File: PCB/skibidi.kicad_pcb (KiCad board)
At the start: 2 copper layers, 99.5 x 79.5 mm, 18 parts, among them J1 Conn_01x05_Pin, SW1 SW_SPDT, SW2 SW_Push, SW3 SW_Push, SW4 SW_Push, SW5 SW_Push, SW6 SW_Push, U1 XIAO-RP2040-DIP

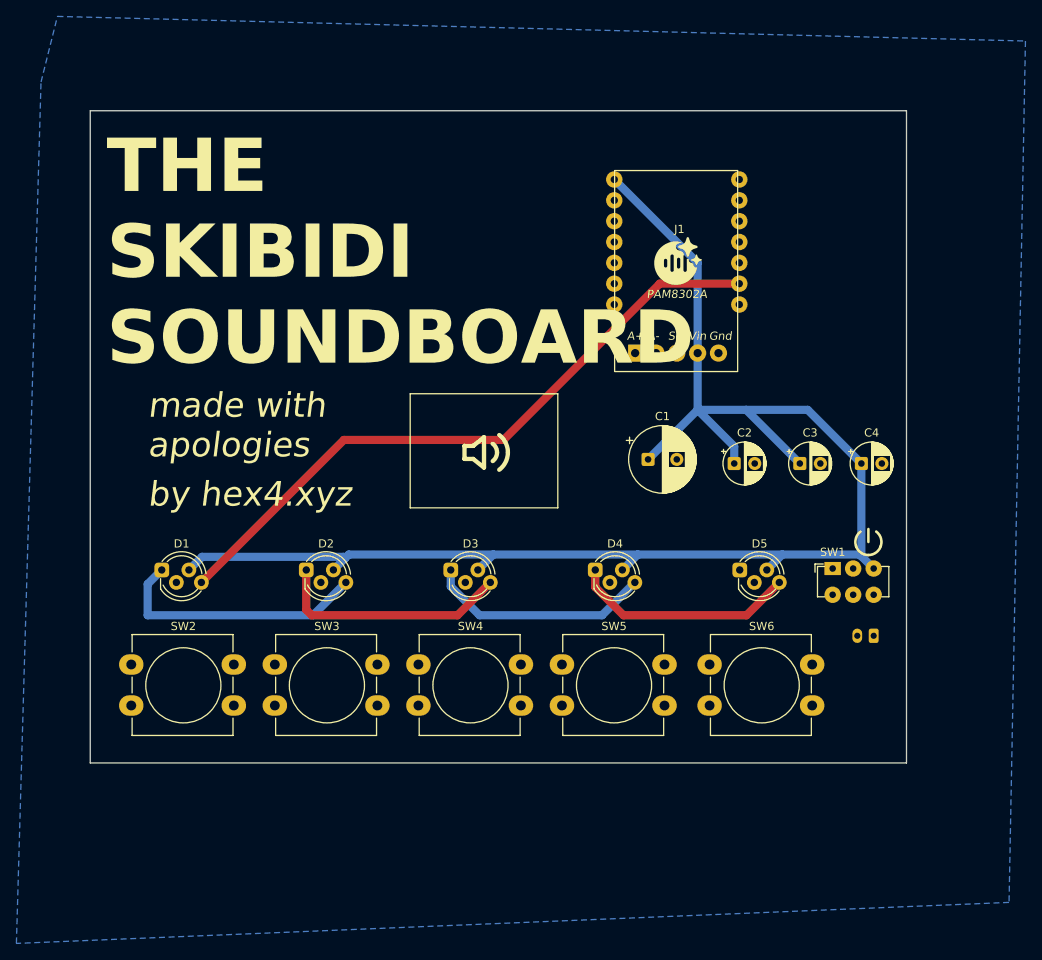
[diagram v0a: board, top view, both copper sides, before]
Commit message: Session 4
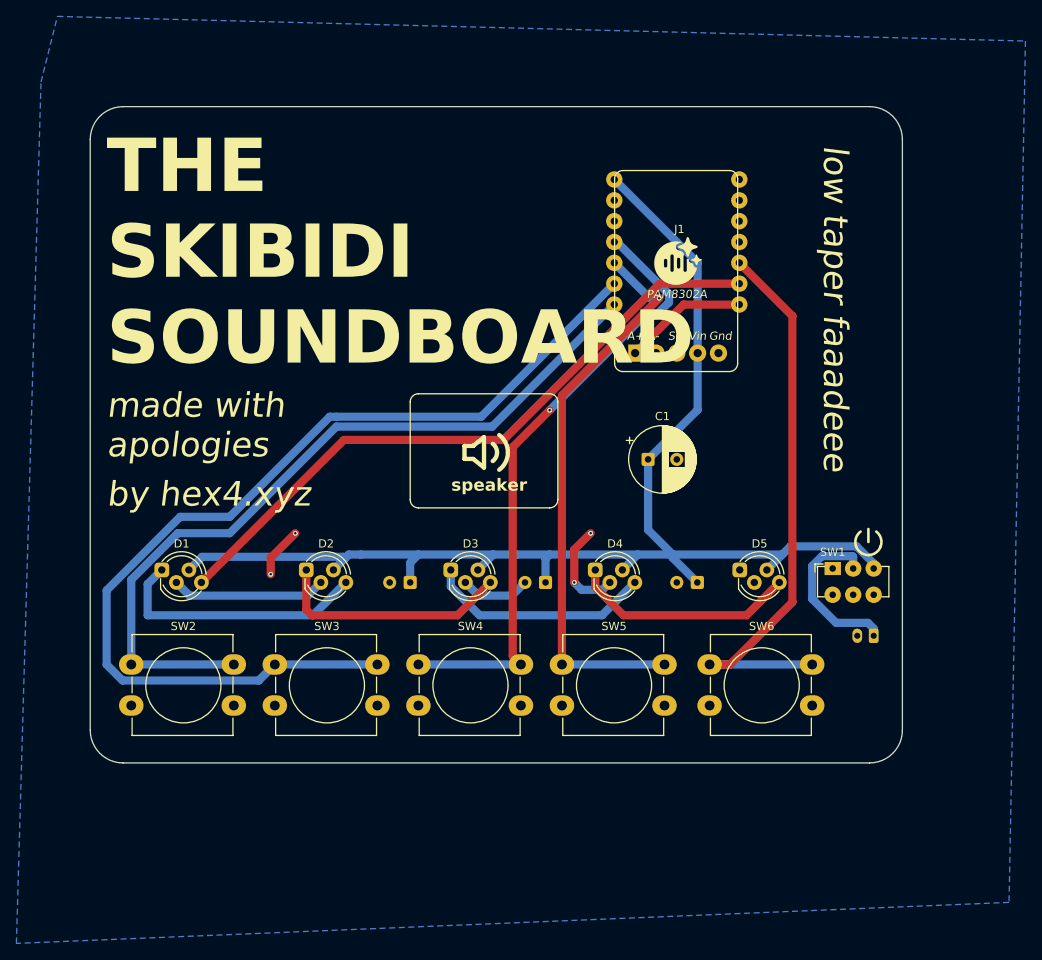
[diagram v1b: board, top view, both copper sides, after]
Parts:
- added G***: LOGO, bad-footprints:tutorial, B.Cu at (143.0, 71.0)
- C2, C3, C4: moved to B.Cu
- moved C2 42.1 mm to (150.0, 95.0), turned to 180 degrees
- moved C3 34.2 mm to (166.5, 95.0), turned to 180 degrees
- moved C4 24.7 mm to (185.0, 95.0), turned to 180 degrees
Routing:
- net BTN2: track 0.00 -> 121.0 mm
- net BTN1: track 0.00 -> 95.6 mm
- net BTN3: track 0.00 -> 76.1 mm, vias 0 -> 1
- net BTN5: track 0.00 -> 69.8 mm
- net BTN4: track 0.00 -> 69.3 mm, vias 0 -> 1
- net GND: track 0.00 -> 45.7 mm, vias 0 -> 4
- net +5V: track 187.5 -> 162.0 mm
- net Net-(BT1-+): track 0.00 -> 20.8 mm
- net A+: track 0.00 -> 15.2 mm
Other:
- board size 99.5 x 79.5 mm -> 99 x 80 mm
- board text added: "erm what the sigma?"
- board text added: "low taper faaadeee"
- board text added: "speaker"
